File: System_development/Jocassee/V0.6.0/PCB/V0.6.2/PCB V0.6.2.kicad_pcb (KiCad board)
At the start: 2 copper layers, 33.5 x 131 mm, 8 parts, among them P1 ST-TF-003A, U1 NRF24L01_Breakout, U2 ProMicro, U3 EZO_PH, U4 EZO_TDS, U5 YAAJ_DCDC_StepDown_LM2596, U6 HX-2S-JH20

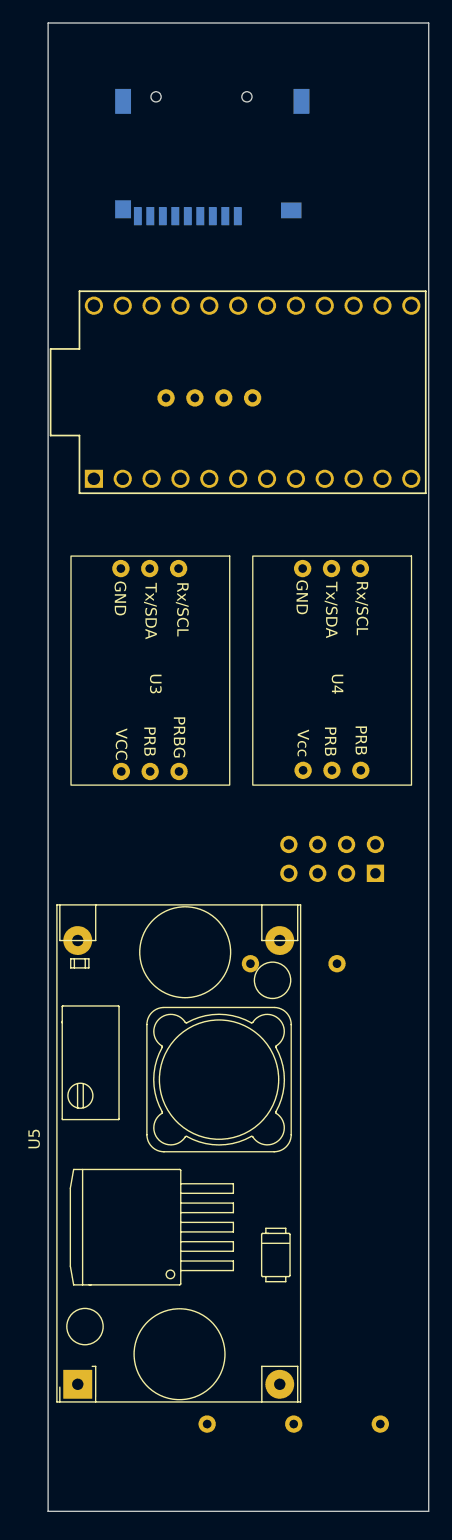
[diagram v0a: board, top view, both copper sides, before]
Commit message: PCB routing done
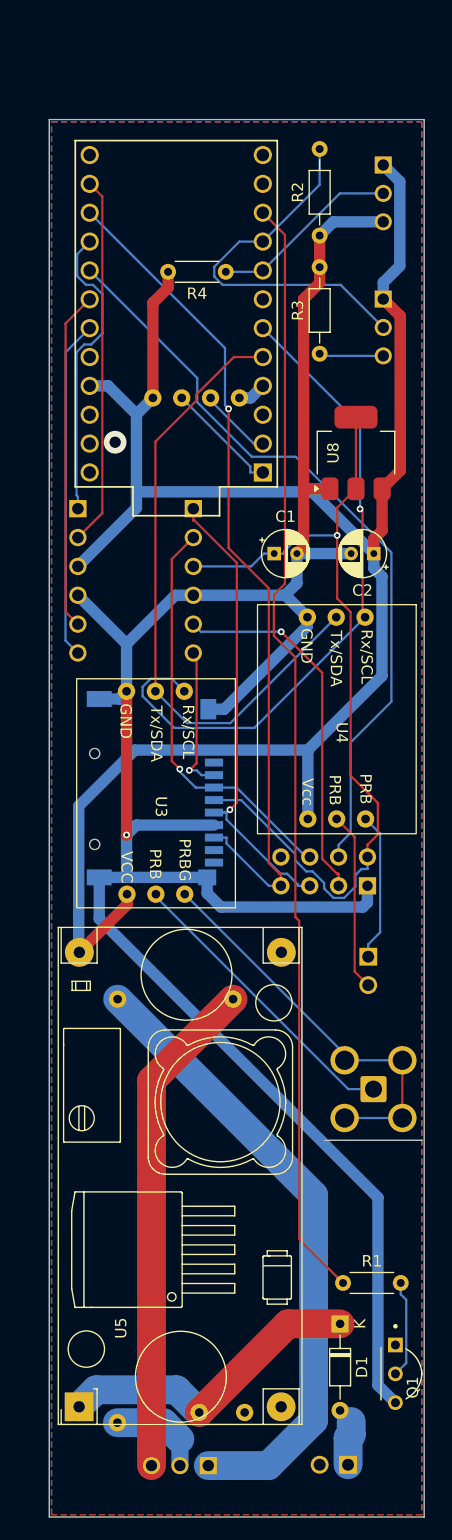
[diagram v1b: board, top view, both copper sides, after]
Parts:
- added C1: C_Polarized, Capacitor_THT:CP_Radial_D4.0mm_P2.00mm, F.Cu at (99.4, 102.2)
- added C2: C_Polarized, Capacitor_THT:CP_Radial_D4.0mm_P2.00mm, F.Cu at (108.2, 102.2)
- added D1: D_Schottky, Diode_THT:D_DO-34_SOD68_P7.62mm_Horizontal, F.Cu at (105.2, 170.0)
- added J1: TDS PRB, XH2.54 - 3pin:JST_B2B-XH-A_LF__SN_, B.Cu at (108.2, 138.9)
- added J2: Temp, XH2.54:XH2.54, B.Cu at (109.5, 70.5)
- added J3: BAT, XH2.54:XH2.54, B.Cu at (91.1, 183.0)
- added J4: TRBDT, XH2.54:XH2.54, B.Cu at (109.5, 82.3)
- added J5: CHRG, XH2.54 - 3pin:JST_B2B-XH-A_LF__SN_, B.Cu at (104.7, 182.9)
- added J6: Conn_Coaxial_Small, Connector_Coaxial:SMA_Amphenol_901-143_Horizontal, B.Cu at (108.1, 149.3)
- added Q1: 2N2222A, 2N2222A:TO92254P470H750-3, F.Cu at (112.4, 174.4)
- added R1: 1K, Resistor_THT:R_Axial_DIN0204_L3.6mm_D1.6mm_P5.08mm_Horizontal, F.Cu at (105.5, 166.4)
- added R2: 4.7K, Resistor_THT:R_Axial_DIN0204_L3.6mm_D1.6mm_P7.62mm_Horizontal, F.Cu at (103.4, 74.2)
- added R3: 470, Resistor_THT:R_Axial_DIN0204_L3.6mm_D1.6mm_P7.62mm_Horizontal, F.Cu at (103.4, 84.6)
- added R4: 4.7K, Resistor_THT:R_Axial_DIN0204_L3.6mm_D1.6mm_P5.08mm_Horizontal, F.Cu at (95.1, 77.4)
- added U7: BOB-12009, Logic level shifter:Logic_level_shifter, B.Cu at (87.2, 104.6)
- added U8: AMS1117 3.3v, Package_TO_SOT_SMD:SOT-223-3_TabPin2, F.Cu at (106.6, 93.3)
- P1: value ST-TF-003A -> SD card socket
- U1: value NRF24L01_Breakout -> NRF24L01+PA+LNA
- U5: value YAAJ_DCDC_StepDown_LM2596 -> DC-DC STPDN LM2596
- U6: value HX-2S-JH20 -> HX-2S-JH10; footprint megasaturnv_custom_components:HX-2S-JH20 -> megasaturnv_custom_components:HX-2S-JH10
- moved P1 57.1 mm to (88.8, 124.1), turned to 90 degrees
- moved U3 10.8 mm to (88.9, 124.5)
- moved U6 10.4 mm to (90.7, 159.2)
- moved U2 9.64 mm to (90.8, 81.1), turned to 90 degrees
- moved U4 4.30 mm to (104.9, 118.0)
- moved U5 1.98 mm to (82.2, 177.3)
- moved U1 1.30 mm to (103.8, 130.2)
- moved M8N_GPS1 1.16 mm to (79.6, 91.5)
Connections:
- M8N_GPS1 pad 1: unconnected-(M8N_GPS1-Vcc-Pad1) -> 5V
- M8N_GPS1 pad 2: unconnected-(M8N_GPS1-RX-Pad2) -> TX
- M8N_GPS1 pad 3: unconnected-(M8N_GPS1-TX-Pad3) -> RX
- M8N_GPS1 pad 4: unconnected-(M8N_GPS1-GND-Pad4) -> GND
- P1 pad 2: unconnected-(P1-DAT3/CS-Pad2) -> Net-(P1-DAT3/CS)
- P1 pad 3: unconnected-(P1-CMD/MOSI-Pad3) -> Net-(P1-CMD/MOSI)
- P1 pad 4: unconnected-(P1-VDD-Pad4) -> 3.3V
- P1 pad 5: unconnected-(P1-CLK/SCK-Pad5) -> Net-(P1-CLK/SCK)
- P1 pad 6: unconnected-(P1-VSS-Pad6) -> V GND
- P1 pad 7: unconnected-(P1-DAT0/MISO-Pad7) -> MISO
- P1 pad G1: Net-(P1-GND-PadG1) -> V GND
- P1 pad G2: Net-(P1-GND-PadG1) -> V GND
- P1 pad G3: Net-(P1-GND-PadG1) -> V GND
- P1 pad G4: Net-(P1-GND-PadG1) -> V GND
- U1 pad 1: unconnected-(U1-GND-Pad1) -> V GND
- U1 pad 2: unconnected-(U1-VCC-Pad2) -> 3.3V
- U1 pad 3: unconnected-(U1-CE-Pad3) -> Net-(U1-CE)
- U1 pad 4: unconnected-(U1-~{CSN}-Pad4) -> NRF CS
- U1 pad 5: unconnected-(U1-SCK-Pad5) -> Net-(P1-CLK/SCK)
- U1 pad 6: unconnected-(U1-MOSI-Pad6) -> Net-(P1-CMD/MOSI)
- U1 pad 7: unconnected-(U1-MISO-Pad7) -> MISO
- U2 pad 1: unconnected-(U2-TX-Pad1) -> TX
- U2 pad 10: unconnected-(U2-E6-Pad10) -> P_EN
- U2 pad 14: unconnected-(U2-B2-Pad14) -> MOSI
- U2 pad 15: unconnected-(U2-B3-Pad15) -> MISO
- U2 pad 16: unconnected-(U2-B1-Pad16) -> SCLK
- U2 pad 17: unconnected-(U2-F7-Pad17) -> NRF CS
- U2 pad 18: unconnected-(U2-F6-Pad18) -> NRF CE
- U2 pad 19: unconnected-(U2-F5-Pad19) -> SD CS
- U2 pad 2: unconnected-(U2-RX-Pad2) -> RX
- U2 pad 21: unconnected-(U2-VCC-Pad21) -> 5V
- U2 pad 23: unconnected-(U2-GND-Pad23) -> GND
- U2 pad 3: unconnected-(U2-GND-Pad3) -> GND
- U2 pad 4: unconnected-(U2-GND-Pad4) -> GND
- U2 pad 5: unconnected-(U2-SDA-Pad5) -> SDA
- U2 pad 6: unconnected-(U2-SCL-Pad6) -> SCL
- U2 pad 8: unconnected-(U2-C6-Pad8) -> Net-(U2-C6)
- U2 pad 9: unconnected-(U2-D7-Pad9) -> Net-(U2-D7)
- U3 pad 1: unconnected-(U3-GND-Pad1) -> V GND
- U3 pad 2: unconnected-(U3-Tx/SDA-Pad2) -> SDA
- U3 pad 3: unconnected-(U3-Rx/SCL-Pad3) -> SCL
- U3 pad 4: unconnected-(U3-Vcc-Pad4) -> 5V
- U3 pad 5: unconnected-(U3-PRB-Pad5) -> Net-(J6-In)
- U3 pad 6: unconnected-(U3-PRBG-Pad6) -> Net-(J6-Ext)
- U4 pad 1: unconnected-(U4-GND-Pad1) -> V GND
- U4 pad 2: unconnected-(U4-Tx/SDA-Pad2) -> SDA
- U4 pad 3: unconnected-(U4-Rx/SCL-Pad3) -> SCL
- U4 pad 4: unconnected-(U4-Vcc-Pad4) -> 5V
- U4 pad 5: unconnected-(U4-PRB-Pad5) -> Net-(J1-Pad2)
- U4 pad 6: unconnected-(U4-PRB-Pad6) -> Net-(J1-Pad1)
- U5 pad 1: unconnected-(U5-Vin-Pad1) -> CHRG rectified
- U5 pad 2: unconnected-(U5-GND-Pad2) -> GND
- U5 pad 3: unconnected-(U5-GND-Pad3) -> GND
- U5 pad 4: unconnected-(U5-Vout-Pad4) -> 5V
- U6 pad 1: unconnected-(U6-P--Pad1) -> GND
- U6 pad 2: unconnected-(U6-P+-Pad2) -> CHRG rectified
- U6 pad 3: unconnected-(U6-B--Pad3) -> BAT -
- U6 pad 4: unconnected-(U6-BM-Pad4) -> BAT M
- U6 pad 5: unconnected-(U6-B+-Pad5) -> BAT+
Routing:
- net V GND: track 0.00 -> 198.7 mm, vias 0 -> 1
- net 5V: track 0.00 -> 162.8 mm
- net P_EN: track 0.00 -> 97.9 mm
- net 3.3V: track 0.00 -> 75.6 mm, vias 0 -> 1
- net MISO: track 0.00 -> 74.2 mm, vias 0 -> 1
- net NRF CS: track 0.00 -> 66.8 mm
- net SCL: track 0.00 -> 59.2 mm, vias 0 -> 1
- net SDA: track 0.00 -> 55.8 mm
- net BAT+: track 0.00 -> 55.1 mm
- net BAT -: track 0.00 -> 44.0 mm
- net Net-(P1-CLK/SCK): track 0.00 -> 41.5 mm, vias 0 -> 1
- net Net-(P1-CMD/MOSI): track 0.00 -> 36.2 mm, vias 0 -> 1
- net Net-(J6-Ext): track 0.00 -> 35.7 mm
- net Net-(U2-D7): track 0.00 -> 33.0 mm
- net Net-(U1-CE): track 0.00 -> 32.5 mm, vias 0 -> 1
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- added copper zone on B.Cu, net GND
- added copper zone on F.Cu, net GND
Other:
- board size 33.5 x 131 mm -> 33 x 123 mm
